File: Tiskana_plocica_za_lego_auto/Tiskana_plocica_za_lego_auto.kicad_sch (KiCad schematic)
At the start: 25 parts, among them J1 Conn_01x16_Pin, J2 Conn_01x20_Pin, M1 Motor_DC, M2 Motor_Servo, U1 L298N, U4 LM2596S-5

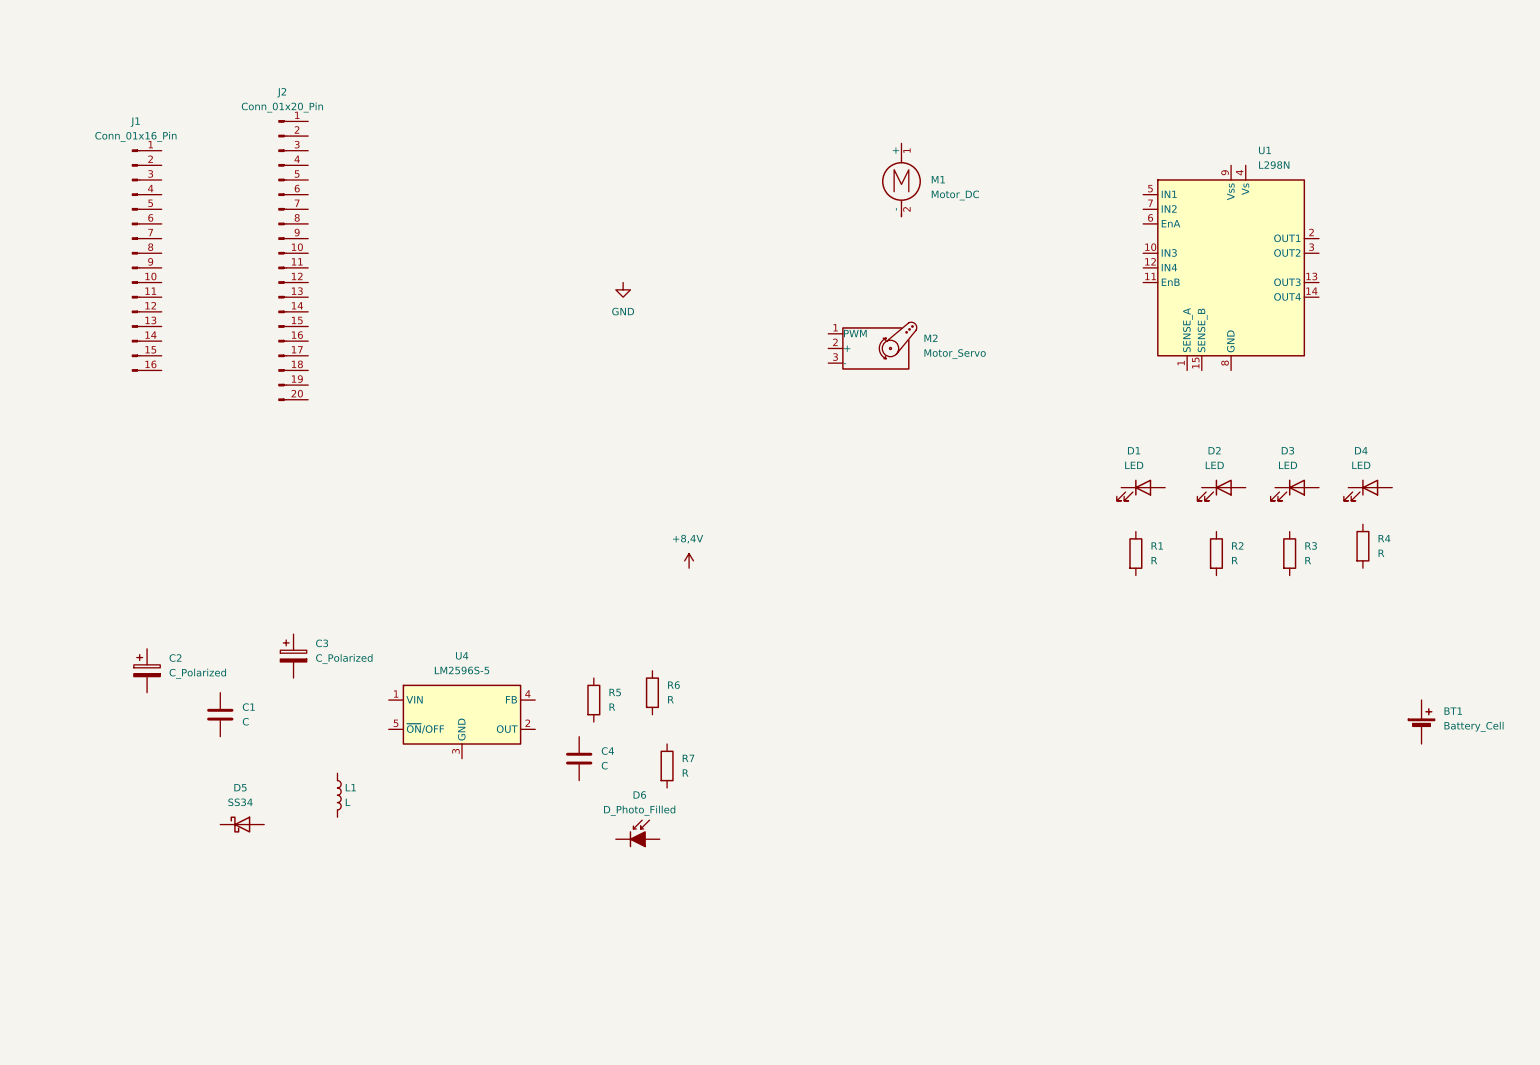
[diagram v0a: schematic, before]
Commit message: seminarskirad2
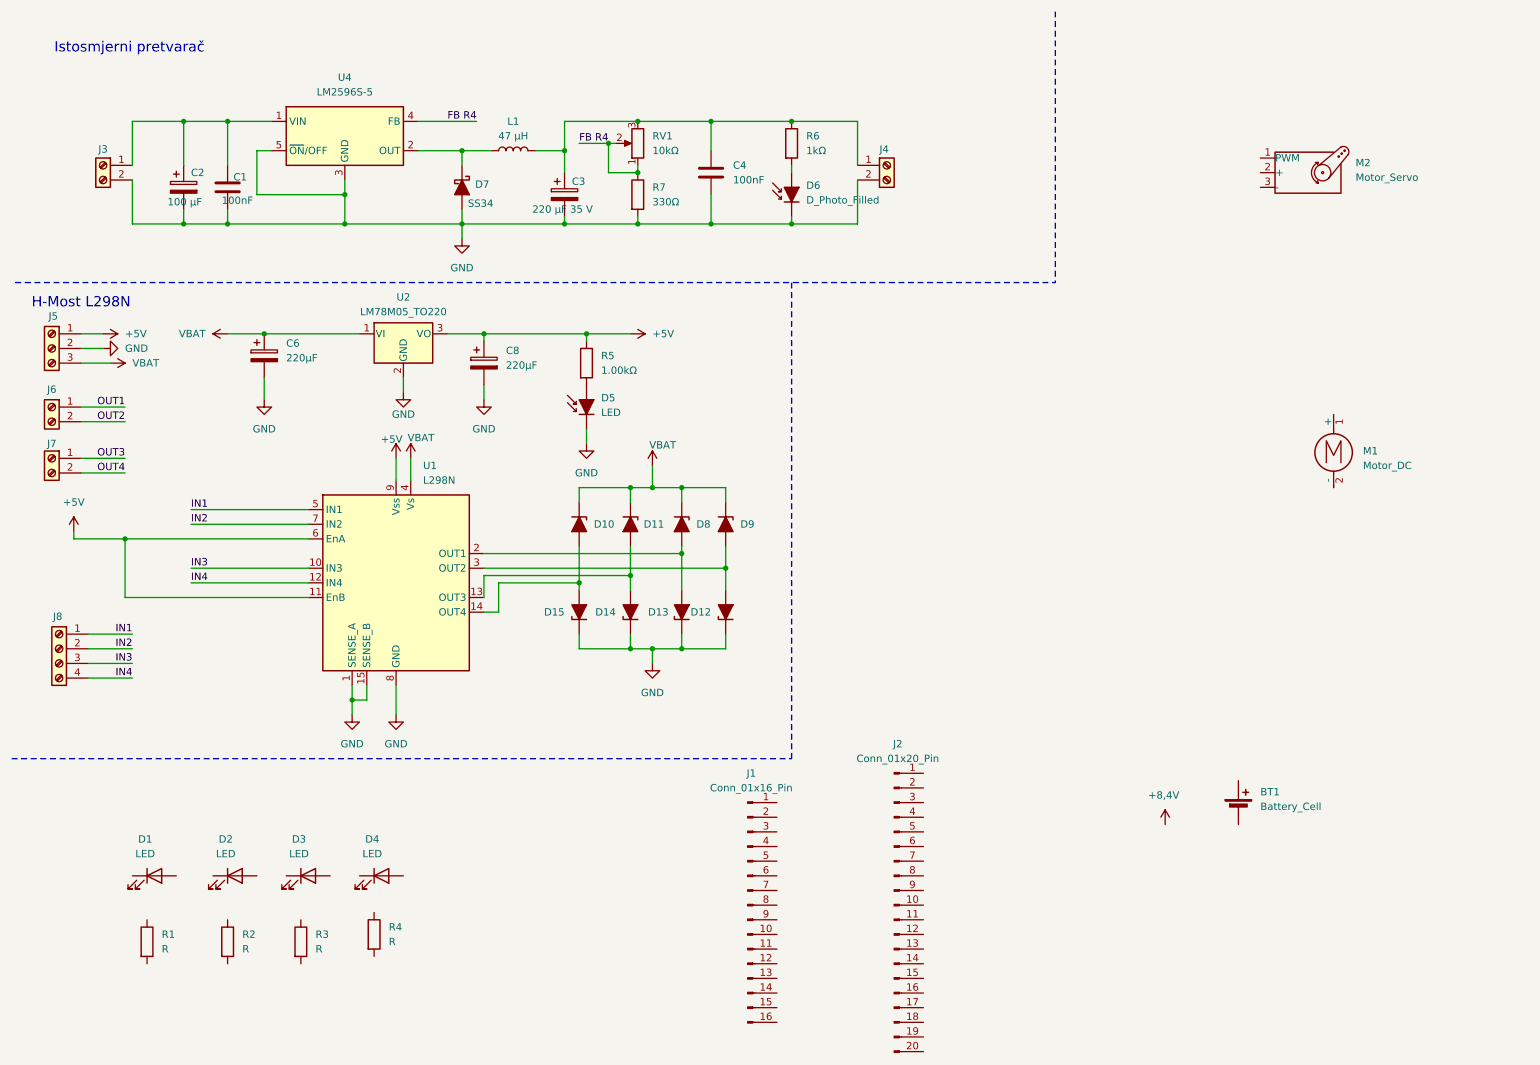
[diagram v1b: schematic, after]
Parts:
- removed D5: SS34, Diode_SMD:D_SMA, symbol Diode:SS34
- added C6, C8: 220μF, symbol Device:C_Polarized
- added D10, D11, D12, D13, D14, D15, D8, D9: D_Zener_Filled, symbol Device:D_Zener_Filled
- added D5: LED, symbol Device:D_Photo_Filled
- added D7: SS34, symbol Device:D_Schottky_Filled
- added J3, J4, J6, J7: Screw_Terminal_01x02, symbol Connector:Screw_Terminal_01x02
- added J5: ~, symbol Connector:Screw_Terminal_01x03
- added J8: Screw_Terminal_01x04, symbol Connector:Screw_Terminal_01x04
- added RV1: 10kΩ, symbol Device:R_Potentiometer
- added U2: LM78M05_TO220, Package_TO_SOT_THT:TO-220-3_Vertical, symbol Regulator_Linear:LM78M05_TO220
- C1, C4: value C -> 100nF
- C2: value C_Polarized -> 100 μF
- C3: value C_Polarized -> 220 μF 35 V
- L1: value L -> 47 μH
- R5: value R -> 1.00kΩ
- R6: value R -> 1kΩ
- R7: value R -> 330Ω
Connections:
- net GND: now also C1.2, C2.2, C3.2, C4.2, D6.1 (K), R7.2, U1.1 (SENSE_A), U1.15 (SENSE_B), U1.8 (GND), U4.3 (GND), U4.5 (~{ON}/OFF), C6.2, C8.2, D12.1 (K), D13.1 (K), D14.1 (K), D15.1 (K), D5.1 (K), D7.2 (A), J3.2 (Pin_2), J4.2 (Pin_2), J5.2 (Pin_2), U2.2 (GND)
- net at L1.1: now also U4.2 (OUT), D7.1 (K)
- net at L1.2: now also C3.1, C4.1, R6.1, J4.1 (Pin_1), RV1.3
- net at R6.2: now also D6.2 (A)
- net +5V: now reaches R5.1
- net +5V: now also U1.11 (EnB), U1.6 (EnA), U1.9 (Vss), C8.1, J5.1 (Pin_1), U2.3 (VO)
- net at R5.2: now also D5.2 (A)
- net IN3: now reaches U1.10 (IN3)
- net IN3: now also J8.3 (Pin_3)
- net IN4: now reaches U1.12 (IN4)
- net IN4: now also J8.4 (Pin_4)
- net at U1.13 (OUT3): now also D11.2 (A), D14.2 (A)
- net at U1.14 (OUT4): now also D10.2 (A), D15.2 (A)
- net at U1.2 (OUT1): now also D13.2 (A), D8.2 (A)
- net at U1.3 (OUT2): now also D12.2 (A), D9.2 (A)
- net VBAT: now reaches U1.4 (Vs)
- net VBAT: now also C6.1, D10.1 (K), D11.1 (K), D8.1 (K), D9.1 (K), J5.3 (Pin_3), U2.1 (VI)
- net IN1: now reaches U1.5 (IN1)
- net IN1: now also J8.1 (Pin_1)
- net IN2: now reaches U1.7 (IN2)
- net IN2: now also J8.2 (Pin_2)
- net at U4.1 (VIN): now also C1.1, C2.1, J3.1 (Pin_1)
- net FB R4: now reaches U4.4 (FB)
- net FB R4: now also R7.1, RV1.1, RV1.2
- new net OUT1: J6.1 (Pin_1)
- new net OUT2: J6.2 (Pin_2)
- new net OUT3: J7.1 (Pin_1)
- new net OUT4: J7.2 (Pin_2)
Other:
- note added: "H-Most L298N"
- note added: "Istosmjerni pretvarač"
- moved on the sheet: BT1, C1, C2, C3, C4, D1, D2, D3, D4, D6, J1, J2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
